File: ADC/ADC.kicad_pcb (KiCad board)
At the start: 2 copper layers, 56.8 x 60.6 mm, 100 parts, among them IC1 ADS7953SDBT, IC2 REF5025ID, IC3 ADS7953SDBT, IC4 REF5025ID, IC5 ADP3338AKCZ-5-REEL, J1 USB_C_Receptacle_USB2.0, J10 Conn_01x04_MountingPin, J11 Conn_01x04_MountingPin, J12 Conn_01x04_MountingPin, J13 Conn_01x04_MountingPin, J14 Conn_01x04_MountingPin, J15 Conn_01x02, J16 Conn_01x02, J2 Conn_01x04_MountingPin, J4 Conn_01x02, J5 Conn_01x02, J6 Conn_01x04_MountingPin, J8 Conn_01x04_MountingPin, J9 Conn_01x04_MountingPin, U1 STM32F072CBT6, U2 OPA192ID, U3 PRTR5V0U2X, U4 XC6206PxxxMR-Regulator_Linear, U5 OPA192ID, U6 SHT4x, U7 LIS3MDL

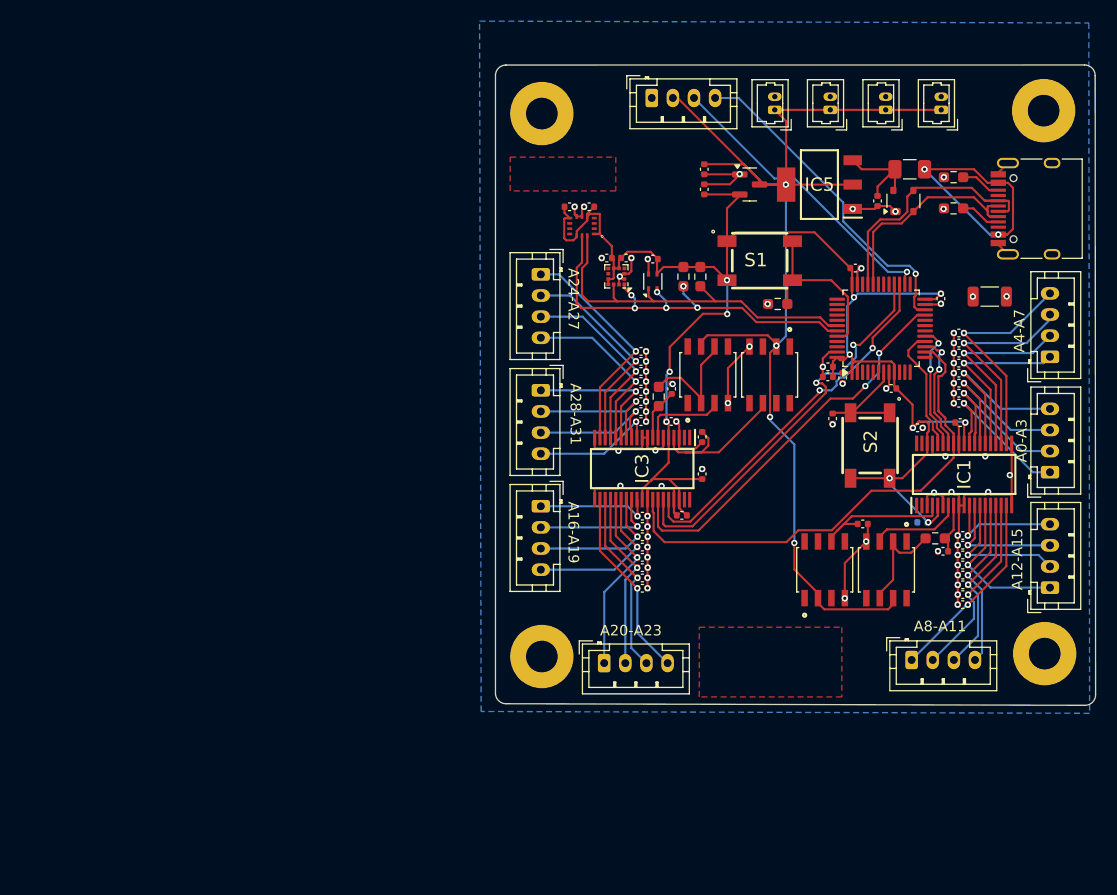
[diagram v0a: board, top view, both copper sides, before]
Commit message: finished V2
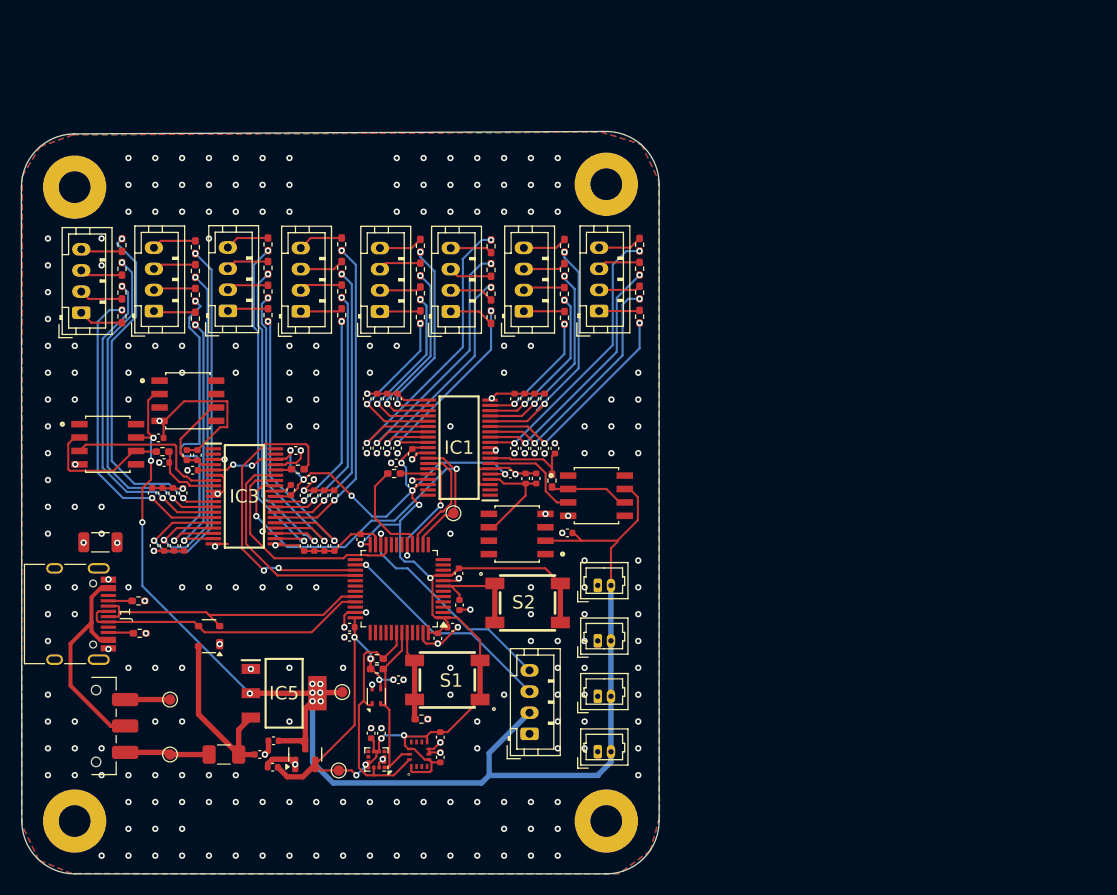
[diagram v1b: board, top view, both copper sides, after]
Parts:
- added C55: 100nF, Capacitor_SMD:C_0402_1005Metric, F.Cu at (70.7, 58.1)
- added C59: 1uF, Capacitor_SMD:C_0402_1005Metric, F.Cu at (73.6, 63.3)
- added C60: 1uF, Capacitor_SMD:C_0402_1005Metric, F.Cu at (34.9, 54.3)
- added C61: 100nF, Capacitor_SMD:C_0402_1005Metric, F.Cu at (57.4, 56.6)
- added C62: 100nF, Capacitor_SMD:C_0402_1005Metric, F.Cu at (49.1, 58.2)
- added C63: 10µF, Capacitor_SMD:C_0402_1005Metric, F.Cu at (37.6, 55.9)
- added R10: 33, Resistor_SMD:R_0402_1005Metric_Pad0.72x0.64mm_HandSolder, F.Cu at (66.4, 38.4)
- added R11: 33, Resistor_SMD:R_0402_1005Metric_Pad0.72x0.64mm_HandSolder, F.Cu at (66.4, 36.1)
- added R12: 33, Resistor_SMD:R_0402_1005Metric_Pad0.72x0.64mm_HandSolder, F.Cu at (59.7, 42.8)
- added R13: 33, Resistor_SMD:R_0402_1005Metric_Pad0.72x0.64mm_HandSolder, F.Cu at (59.7, 40.6)
- added R14: 33, Resistor_SMD:R_0402_1005Metric_Pad0.72x0.64mm_HandSolder, F.Cu at (59.7, 38.3)
- added R15: 33, Resistor_SMD:R_0402_1005Metric_Pad0.72x0.64mm_HandSolder, F.Cu at (59.7, 36.1)
- added R16: 33, Resistor_SMD:R_0402_1005Metric_Pad0.72x0.64mm_HandSolder, F.Cu at (73.3, 42.9)
- added R17: 33, Resistor_SMD:R_0402_1005Metric_Pad0.72x0.64mm_HandSolder, F.Cu at (73.3, 40.6)
- added R18: 33, Resistor_SMD:R_0402_1005Metric_Pad0.72x0.64mm_HandSolder, F.Cu at (73.3, 38.4)
- added R19: 33, Resistor_SMD:R_0402_1005Metric_Pad0.72x0.64mm_HandSolder, F.Cu at (73.3, 36.1)
- added R20: 33, Resistor_SMD:R_0402_1005Metric_Pad0.72x0.64mm_HandSolder, F.Cu at (80.5, 42.8)
- added R21: 33, Resistor_SMD:R_0402_1005Metric_Pad0.72x0.64mm_HandSolder, F.Cu at (80.5, 40.5)
- added R22: 33, Resistor_SMD:R_0402_1005Metric_Pad0.72x0.64mm_HandSolder, F.Cu at (80.5, 38.3)
- added R23: 33, Resistor_SMD:R_0402_1005Metric_Pad0.72x0.64mm_HandSolder, F.Cu at (80.5, 36.0)
- added R24: 33, Resistor_SMD:R_0402_1005Metric_Pad0.72x0.64mm_HandSolder, F.Cu at (52.2, 42.7)
- added R25: 33, Resistor_SMD:R_0402_1005Metric_Pad0.72x0.64mm_HandSolder, F.Cu at (52.2, 40.4)
- added R26: 33, Resistor_SMD:R_0402_1005Metric_Pad0.72x0.64mm_HandSolder, F.Cu at (52.2, 38.2)
- added R27: 33, Resistor_SMD:R_0402_1005Metric_Pad0.72x0.64mm_HandSolder, F.Cu at (52.2, 36.0)
- added R28: 33, Resistor_SMD:R_0402_1005Metric_Pad0.72x0.64mm_HandSolder, F.Cu at (45.3, 42.6)
- added R29: 33, Resistor_SMD:R_0402_1005Metric_Pad0.72x0.64mm_HandSolder, F.Cu at (45.3, 40.4)
- added R30: 33, Resistor_SMD:R_0402_1005Metric_Pad0.72x0.64mm_HandSolder, F.Cu at (45.3, 38.2)
- added R31: 33, Resistor_SMD:R_0402_1005Metric_Pad0.72x0.64mm_HandSolder, F.Cu at (45.3, 36.0)
- added R32: 33, Resistor_SMD:R_0402_1005Metric_Pad0.72x0.64mm_HandSolder, F.Cu at (38.4, 43.0)
- added R33: 33, Resistor_SMD:R_0402_1005Metric_Pad0.72x0.64mm_HandSolder, F.Cu at (38.4, 40.7)
- added R34: 33, Resistor_SMD:R_0402_1005Metric_Pad0.72x0.64mm_HandSolder, F.Cu at (38.4, 38.5)
- added R35: 33, Resistor_SMD:R_0402_1005Metric_Pad0.72x0.64mm_HandSolder, F.Cu at (38.4, 36.2)
- added R36: 33, Resistor_SMD:R_0402_1005Metric_Pad0.72x0.64mm_HandSolder, F.Cu at (31.4, 42.8)
- added R37: 33, Resistor_SMD:R_0402_1005Metric_Pad0.72x0.64mm_HandSolder, F.Cu at (31.4, 40.5)
- added R38: 33, Resistor_SMD:R_0402_1005Metric_Pad0.72x0.64mm_HandSolder, F.Cu at (31.4, 38.3)
- added R39: 33, Resistor_SMD:R_0402_1005Metric_Pad0.72x0.64mm_HandSolder, F.Cu at (31.4, 36.0)
- added R40: 33, Resistor_SMD:R_0402_1005Metric_Pad0.72x0.64mm_HandSolder, F.Cu at (57.2, 57.6)
- added R41: 33, Resistor_SMD:R_0402_1005Metric_Pad0.72x0.64mm_HandSolder, F.Cu at (48.1, 57.2)
- added R8: 33, Resistor_SMD:R_0402_1005Metric_Pad0.72x0.64mm_HandSolder, F.Cu at (66.4, 42.8)
- added R9: 33, Resistor_SMD:R_0402_1005Metric_Pad0.72x0.64mm_HandSolder, F.Cu at (66.4, 40.6)
- added SW1: SW_SPDT, Button_Switch_SMD:SW_SPDT_CK_JS102011SAQN, F.Cu at (29.0, 81.5)
- added TP10: TestPoint, TestPoint:TestPoint_Pad_D1.0mm, F.Cu at (52.3, 78.3)
- added TP11: TestPoint, TestPoint:TestPoint_Pad_D1.0mm, F.Cu at (36.0, 79.0)
- added TP12: TestPoint, TestPoint:TestPoint_Pad_D1.0mm, F.Cu at (36.0, 84.2)
- added TP4: TestPoint, TestPoint:TestPoint_Pad_D1.0mm, F.Cu at (62.8, 61.4)
- added TP9: TestPoint, TestPoint:TestPoint_Pad_D1.0mm, F.Cu at (52.0, 85.8)
- C1: value 1µF -> 100nF; moved to F.Cu
- C13, C14, C15, C16, C17, C18, C19, C20, C21, C22, C23, C24, C25, C26, C27, C28, C29, C30, C31, C32, C34, C35, C36, C37, C38, C39, C40, C41, C43, C44, C45, C46, C47, C48: value 150pF -> 270pF
- C2: value 1µF -> 100nF
- C50, C51: value 1µF -> 10uF
- C52: value 10µF -> 100nF
- G***: moved to F.Cu
- R1, R2, R3, R6, R7: footprint Resistor_SMD:R_0603_1608Metric_Pad0.98x0.95mm_HandSolder -> Resistor_SMD:R_0402_1005Metric_Pad0.72x0.64mm_HandSolder
- R4, R5: value 100 -> 33; footprint Resistor_SMD:R_0603_1608Metric_Pad0.98x0.95mm_HandSolder -> Resistor_SMD:R_0402_1005Metric_Pad0.72x0.64mm_HandSolder
- moved H1 113.7 mm to (27.0, 90.5)
- moved J1 100.0 mm to (26.1, 71.0), turned to -90 degrees
- moved R3 88.3 mm to (33.1, 72.8), turned to 180 degrees
- moved L1 87.3 mm to (29.4, 64.2), turned to 180 degrees
- moved R2 85.6 mm to (33.0, 69.7), turned to 180 degrees
- moved F1 85.3 mm to (41.1, 84.2), turned to 0 degrees
- moved C10 78.5 mm to (44.5, 84.2), turned to 0 degrees
- moved U3 77.6 mm to (39.7, 73.0), turned to 180 degrees
- moved IC5 69.9 mm to (46.8, 78.5), turned to 0 degrees
- moved J16 68.9 mm to (76.5, 84.0), turned to 0 degrees
- moved U4 68.4 mm to (48.8, 84.2), turned to 90 degrees
- moved C12 68.3 mm to (45.7, 85.5), turned to 0 degrees
- moved C11 67.7 mm to (45.8, 83.0), turned to 0 degrees
- moved J8 63.6 mm to (55.9, 42.3)
- moved H2 62.7 mm to (27.0, 30.5)
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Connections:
- F1 pad 1: VBUS -> VBUS_IN
- H4 pad 1: (no net) -> GND
- IC1 pad 34: MISO_SPI1 -> Net-(IC1-SDO)
- IC3 pad 34: MISO_SPI2 -> Net-(IC3-SDO)
- J10 pad 1: A12 -> Net-(J10-Pin_1)
- J10 pad 2: A13 -> Net-(J10-Pin_2)
- J10 pad 3: A14 -> Net-(J10-Pin_3)
- J10 pad 4: A15 -> Net-(J10-Pin_4)
- J11 pad 1: A20 -> Net-(J11-Pin_1)
- J11 pad 2: A21 -> Net-(J11-Pin_2)
- J11 pad 3: A22 -> Net-(J11-Pin_3)
- J11 pad 4: A23 -> Net-(J11-Pin_4)
- J12 pad 1: A16 -> Net-(J12-Pin_1)
- J12 pad 2: A17 -> Net-(J12-Pin_2)
- J12 pad 3: A18 -> Net-(J12-Pin_3)
- J12 pad 4: A19 -> Net-(J12-Pin_4)
- J13 pad 1: A24 -> Net-(J13-Pin_1)
- J13 pad 2: A25 -> Net-(J13-Pin_2)
- J13 pad 3: A26 -> Net-(J13-Pin_3)
- J13 pad 4: A27 -> Net-(J13-Pin_4)
- J14 pad 1: A28 -> Net-(J14-Pin_1)
- J14 pad 2: A29 -> Net-(J14-Pin_2)
- J14 pad 3: A30 -> Net-(J14-Pin_3)
- J14 pad 4: A31 -> Net-(J14-Pin_4)
- J15 pad 1: +5V -> GND
- J15 pad 2: GND -> +5V
- J16 pad 1: +5V -> GND
- J16 pad 2: GND -> +5V
- J2 pad 1: A0 -> Net-(J2-Pin_1)
- J2 pad 2: A1 -> Net-(J2-Pin_2)
- J2 pad 3: A2 -> Net-(J2-Pin_3)
- J2 pad 4: A3 -> Net-(J2-Pin_4)
- J4 pad 1: +5V -> GND
- J4 pad 2: GND -> +5V
- J5 pad 1: +5V -> GND
- J5 pad 2: GND -> +5V
- J8 pad 1: A4 -> Net-(J8-Pin_1)
- J8 pad 2: A5 -> Net-(J8-Pin_2)
- J8 pad 3: A6 -> Net-(J8-Pin_3)
- J8 pad 4: A7 -> Net-(J8-Pin_4)
- J9 pad 1: A8 -> Net-(J9-Pin_1)
- J9 pad 2: A9 -> Net-(J9-Pin_2)
- J9 pad 3: A10 -> Net-(J9-Pin_3)
- J9 pad 4: A11 -> Net-(J9-Pin_4)
- U1 pad 10: /PA0 -> unconnected-(U1-PA0-Pad10)
- U1 pad 11: /PA1 -> unconnected-(U1-PA1-Pad11)
- U1 pad 12: /PA2 -> unconnected-(U1-PA2-Pad12)
- U1 pad 13: /PA3 -> unconnected-(U1-PA3-Pad13)
- U1 pad 18: /PB0 -> unconnected-(U1-PB0-Pad18)
- U1 pad 19: /PB1 -> unconnected-(U1-PB1-Pad19)
- U1 pad 2: /PC13 -> unconnected-(U1-PC13-Pad2)
- U1 pad 20: /PB2 -> unconnected-(U1-PB2-Pad20)
- U1 pad 25: /PB12 -> unconnected-(U1-PB12-Pad25)
- U1 pad 29: /PA8 -> unconnected-(U1-PA8-Pad29)
- U1 pad 3: /PC14 -> unconnected-(U1-PC14-Pad3)
- U1 pad 30: /PA9 -> unconnected-(U1-PA9-Pad30)
- U1 pad 31: /PA10 -> unconnected-(U1-PA10-Pad31)
- U1 pad 34: /PA13 -> unconnected-(U1-PA13-Pad34)
- U1 pad 37: /PA14 -> unconnected-(U1-PA14-Pad37)
- U1 pad 38: /PA15 -> unconnected-(U1-PA15-Pad38)
- U1 pad 39: /PB3 -> unconnected-(U1-PB3-Pad39)
- U1 pad 4: /PC15 -> unconnected-(U1-PC15-Pad4)
- U1 pad 40: /PB4 -> unconnected-(U1-PB4-Pad40)
- U1 pad 41: /PB5 -> unconnected-(U1-PB5-Pad41)
- U1 pad 45: /PB8 -> unconnected-(U1-PB8-Pad45)
- U1 pad 46: /PB9 -> unconnected-(U1-PB9-Pad46)
- U1 pad 5: /PF0 -> unconnected-(U1-PF0-Pad5)
- U1 pad 6: /PF1 -> unconnected-(U1-PF1-Pad6)
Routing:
- net GND: track 135.3 -> 97.6 mm, vias 71 -> 259
- net +5V: track 111.6 -> 135.5 mm, vias 4 -> 10
- net A27: track 16.8 -> 39.7 mm, vias 1 -> 2
- net A31: track 11.8 -> 34.2 mm, vias 1 -> 2
- net SCL_I2C1: track 39.9 -> 17.6 mm, vias 6 -> 0
- net A30: track 12.6 -> 32.3 mm, vias 1 -> 2
- net MOSI_SPI2: track 38.4 -> 20.4 mm, vias 2 -> 0
- net A29: track 13.5 -> 30.7 mm, vias 1 -> 2
- net A19: track 15.1 -> 31.3 mm, vias 1 -> 2
- net A26: track 18.5 -> 34.5 mm, vias 1 -> 2
- net A28: track 14.0 -> 29.8 mm, vias 1 -> 2
- net SCK_SPI2: track 37.5 -> 22.0 mm, vias 2 -> 0
- net A15: track 11.1 -> 26.2 mm, vias 1 -> 2
- net A23: track 18.1 -> 33.0 mm, vias 1 -> 2
- net A22: track 17.6 -> 32.3 mm, vias 1 -> 2
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- added copper zone on F.Cu, net GND
- removed copper zone on F.Cu, net (none)
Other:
- board size 56.8 x 60.6 mm -> 60.4 x 70.3 mm
- board text removed: "A0-A3"
- board text removed: "A12-A15"
- board text removed: "A16-A19"
- board text removed: "A20-A23"
- board text removed: "A24-A27"
- board text removed: "A28-A31"
- board text removed: "A4-A7"
- board text removed: "A8-A11"
